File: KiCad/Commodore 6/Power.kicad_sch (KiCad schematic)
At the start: 33 parts, among them J6 6130XX11121_61300511121, Q1 NTR4501NT1G, Q2 PMOS

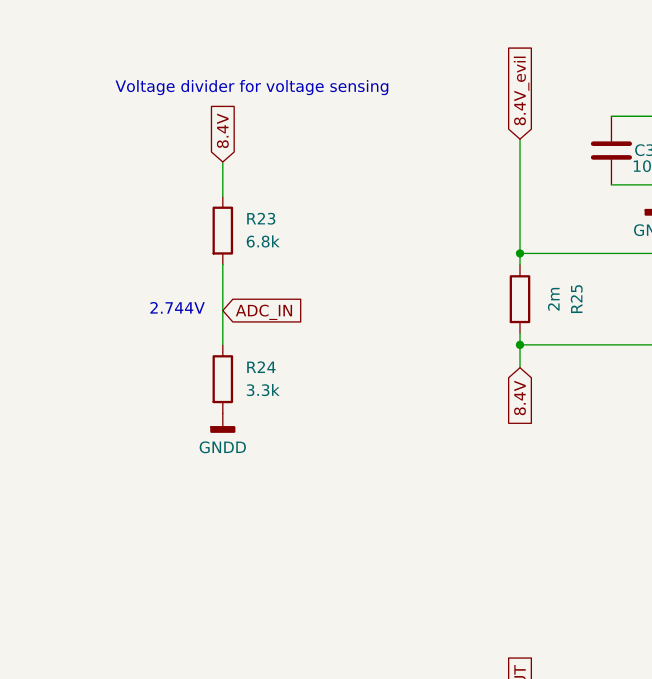
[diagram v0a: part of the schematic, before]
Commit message: chud
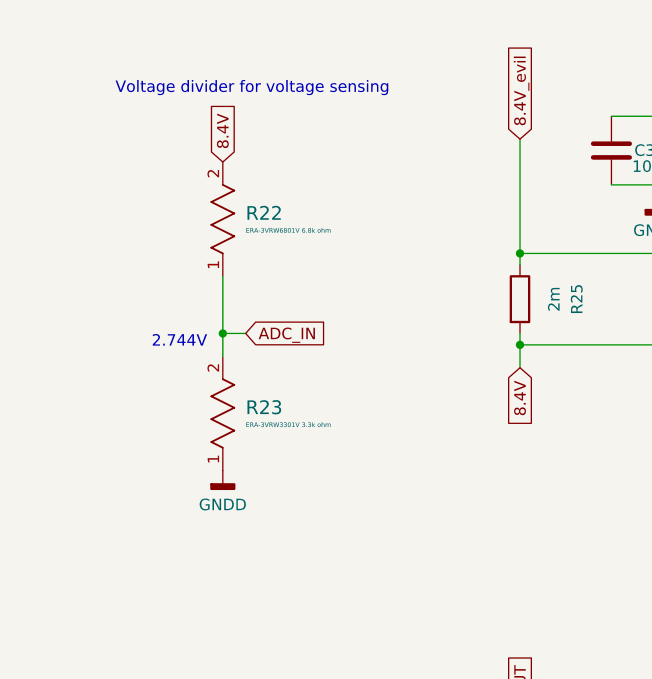
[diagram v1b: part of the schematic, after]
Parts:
- removed R23: 6.8k, symbol Device:R
- removed R24: 3.3k, symbol Device:R
- added R22: ERA-3VRW6801V 6.8k ohm, RES_ERA3V_3K_PAN, symbol 2025-10-26_23-22-38:ERA-3VRW6801V
- added R23: ERA-3VRW3301V 3.3k ohm, RES_ERA3V_3K_PAN, symbol 2025-10-26_23-30-03:ERA-3VRW3301V
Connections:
- net 8.4V: now also R22.2
- net ADC_IN: now also R22.1, R23.2
- net GNDD: now also R23.1
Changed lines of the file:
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@@
 	(text "2.744V\n"
 		(exclude_from_sim no)
-		(at 26.67 93.98 0)
+		(at 26.924 97.536 0)
 		(effects
 			(font
@@
 	)
 	(junction
+		(at 31.75 96.52)
+		(diameter 0)
+		(color 0 0 0 0)
+	)
+	(junction
 		(at 93.98 72.39)
 		(diameter 0)
@@
 	(wire
 		(pts
-			(xy 31.75 77.47) (xy 31.75 81.28)
+			(xy 31.75 96.52) (xy 31.75 99.06)
 		)
 		(stroke
@@
 	(wire
 		(pts
-			(xy 31.75 97.79) (xy 31.75 88.9)
+			(xy 34.29 96.52) (xy 31.75 96.52)
 		)
 		(stroke
@@
 	(wire
 		(pts
+			(xy 31.75 90.17) (xy 31.75 96.52)
+		)
+		(stroke
+			(width 0)
+			(type default)
+		)
+	)
+	(wire
+		(pts
 			(xy 64.77 87.63) (xy 83.82 87.63)
 		)
@@
 	(global_label "ADC_IN"
 		(shape input)
-		(at 31.75 93.98 0)
+		(at 34.29 96.52 0)
 		(fields_autoplaced yes)
 		(effects
@@
 		)
 		(property "Intersheetrefs" "${INTERSHEET_REFS}"
-			(at 41.2667 93.98 0)
+			(at 43.8067 96.52 0)
 			(effects
 				(font
@@
 	)
 	(symbol
-		(lib_id "Device:R")
-		(at 31.75 101.6 0)
+		(lib_id "2025-10-26_23-30-03:ERA-3VRW3301V")
+		(at 31.75 111.76 90)
 		(unit 1)
 		(exclude_from_sim no)
@@
 		(dnp no)
 		(fields_autoplaced yes)
-		(property "Reference" "R24"
-			(at 34.29 100.3299 0)
+		(property "Reference" "R23"
+			(at 34.29 104.7749 90)
 			(effects
 				(font
-					(size 1.27 1.27)
+					(size 1.524 1.524)
 				)
-				(justify left)
+				(justify right)
 			)
 		)
-		(property "Value" "3.3k"
-			(at 34.29 102.8699 0)
+		(property "Value" "ERA-3VRW3301V 3.3k ohm"
+			(at 34.29 106.68 90)
 			(effects
 				(font
-					(size 1.27 1.27)
+					(size 0.508 0.508)
 				)
-				(justify left)
+				(justify right)
 			)
 		)
-		(property "Footprint" ""
-			(at 29.972 101.6 90)
+		(property "Footprint" "RES_ERA3V_3K_PAN"
+			(at 31.75 111.76 0)
 			(effects
 				(font
 					(size 1.27 1.27)
+					(italic yes)
 				)
 				(hide yes)
 			)
 		)
-		(property "Datasheet" "~"
-			(at 31.75 101.6 0)
+		(property "Datasheet" "ERA-3VRW3301V"
+			(at 31.75 111.76 0)
 			(effects
 				(font
 					(size 1.27 1.27)
+					(italic yes)
 				)
 				(hide yes)
 			)
 		)
-		(property "Description" "Resistor"
-			(at 31.75 101.6 0)
+		(property "Description" ""
+			(at 31.75 111.76 0)
 			(effects
 				(font
@@
 		)
 		(instances
-			(project "Commodore 6"
+			(project ""
 				(path "/27ad1105-577c-4f6a-be9a-9e41c9021a88/0eaef56c-69f1-4e48-a682-2dae5a86159f"
-					(reference "R24")
+					(reference "R23")
 					(unit 1)
 				)
@@
 	)
 	(symbol
-		(lib_id "Device:R")
-		(at 31.75 85.09 0)
+		(lib_id "2025-10-26_23-22-38:ERA-3VRW6801V")
+		(at 31.75 90.17 90)
 		(unit 1)
 		(exclude_from_sim no)
@@
 		(dnp no)
 		(fields_autoplaced yes)
-		(property "Reference" "R23"
-			(at 34.29 83.8199 0)
+		(property "Reference" "R22"
+			(at 34.29 83.1849 90)
 			(effects
 				(font
-					(size 1.27 1.27)
+					(size 1.524 1.524)
 				)
-				(justify left)
+				(justify right)
 			)
 		)
-		(property "Value" "6.8k"
-			(at 34.29 86.3599 0)
+		(property "Value" "ERA-3VRW6801V 6.8k ohm"
+			(at 34.29 85.09 90)
 			(effects
 				(font
-					(size 1.27 1.27)
+					(size 0.508 0.508)
 				)
-				(justify left)
+				(justify right)
 			)
 		)
-		(property "Footprint" ""
-			(at 29.972 85.09 90)
+		(property "Footprint" "RES_ERA3V_3K_PAN"
+			(at 31.75 90.17 0)
 			(effects
 				(font
 					(size 1.27 1.27)
+					(italic yes)
 				)
 				(hide yes)
 			)
 		)
-		(property "Datasheet" "~"
-			(at 31.75 85.09 0)
+		(property "Datasheet" "ERA-3VRW6801V"
+			(at 31.75 90.17 0)
 			(effects
 				(font
 					(size 1.27 1.27)
+					(italic yes)
 				)
 				(hide yes)
 			)
 		)
-		(property "Description" "Resistor"
-			(at 31.75 85.09 0)
+		(property "Description" ""
+			(at 31.75 90.17 0)
 			(effects
 				(font
@@
 			(project ""
 				(path "/27ad1105-577c-4f6a-be9a-9e41c9021a88/0eaef56c-69f1-4e48-a682-2dae5a86159f"
-					(reference "R23")
+					(reference "R22")
 					(unit 1)
 				)
@@
 	(symbol
 		(lib_id "power:GNDD")
-		(at 31.75 105.41 0)
+		(at 31.75 111.76 0)
 		(unit 1)
 		(exclude_from_sim no)
@@
 		(fields_autoplaced yes)
 		(property "Reference" "#PWR095"
-			(at 31.75 111.76 0)
+			(at 31.75 118.11 0)
 			(effects
 				(font
@@
 		)
 		(property "Value" "GNDD"
-			(at 31.75 109.22 0)
+			(at 31.75 115.57 0)
 			(effects
 				(font
@@
 		)
 		(property "Footprint" ""
-			(at 31.75 105.41 0)
+			(at 31.75 111.76 0)
 			(effects
 				(font
@@
 		)
 		(property "Datasheet" ""
-			(at 31.75 105.41 0)
+			(at 31.75 111.76 0)
 			(effects
 				(font
@@
 		)
 		(property "Description" "Power symbol creates a global label with name \"GNDD\" , digital ground"
-			(at 31.75 105.41 0)
+			(at 31.75 111.76 0)
 			(effects
 				(font
